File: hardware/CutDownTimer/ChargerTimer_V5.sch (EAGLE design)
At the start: 50 parts, among them Q1 2N3906, Q3 2N3906, Q4 2N3906, T1 2N3904, T2 2N3904, T4 2N3904, U1 ADCMP354OC, U2 ADCMP354OC, U3 LM60

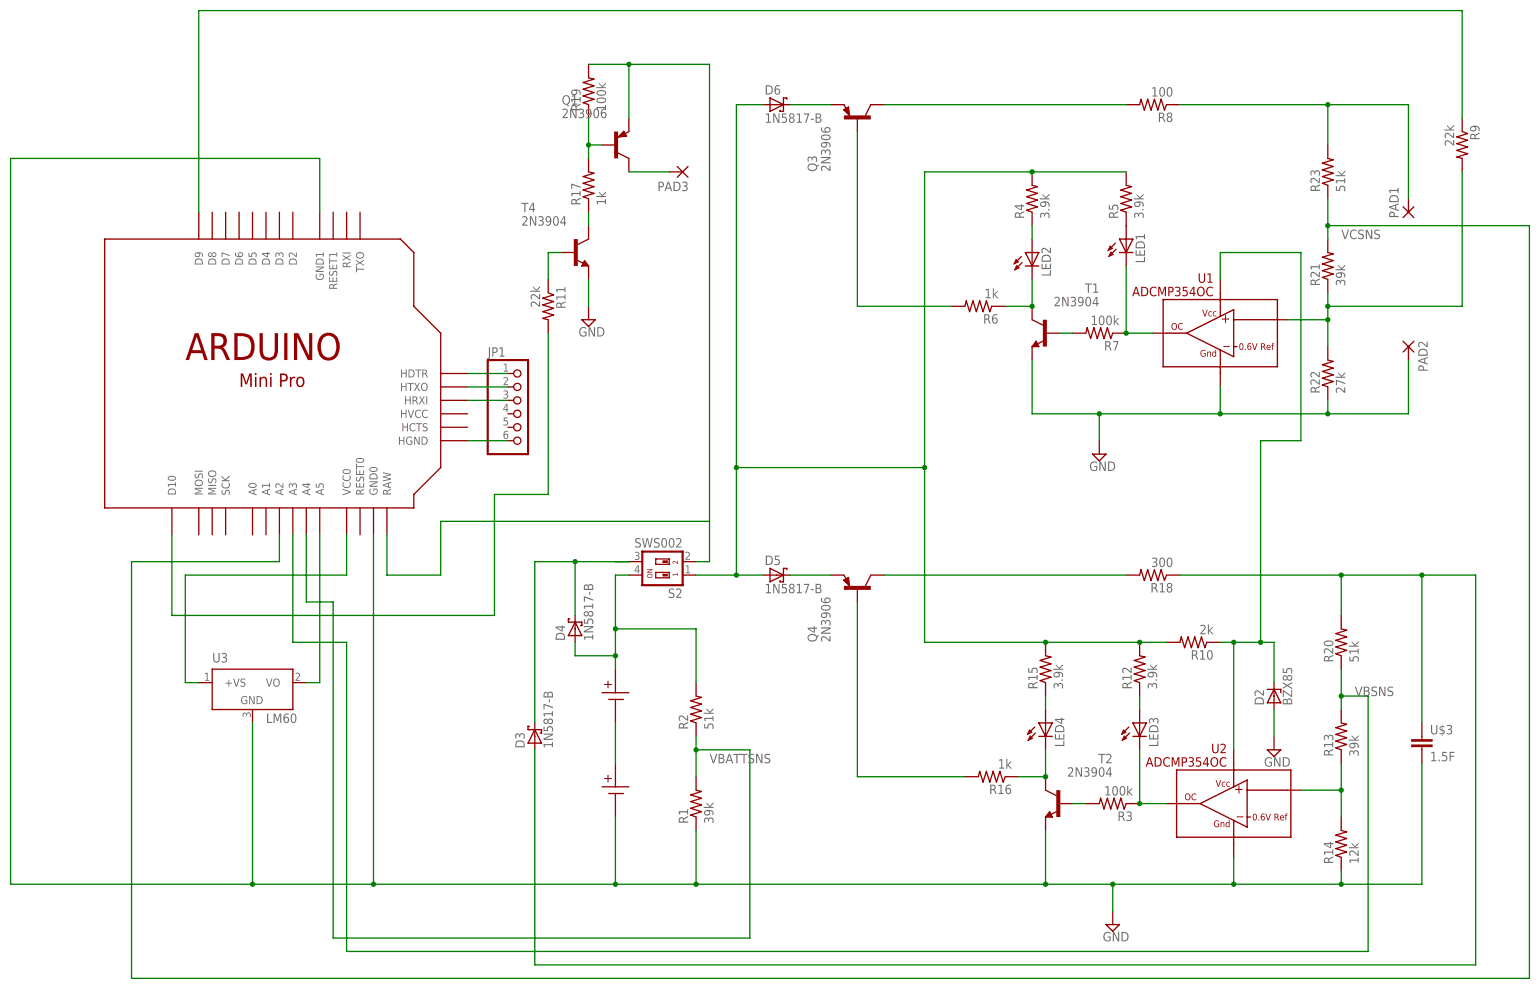
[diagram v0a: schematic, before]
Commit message: Updates
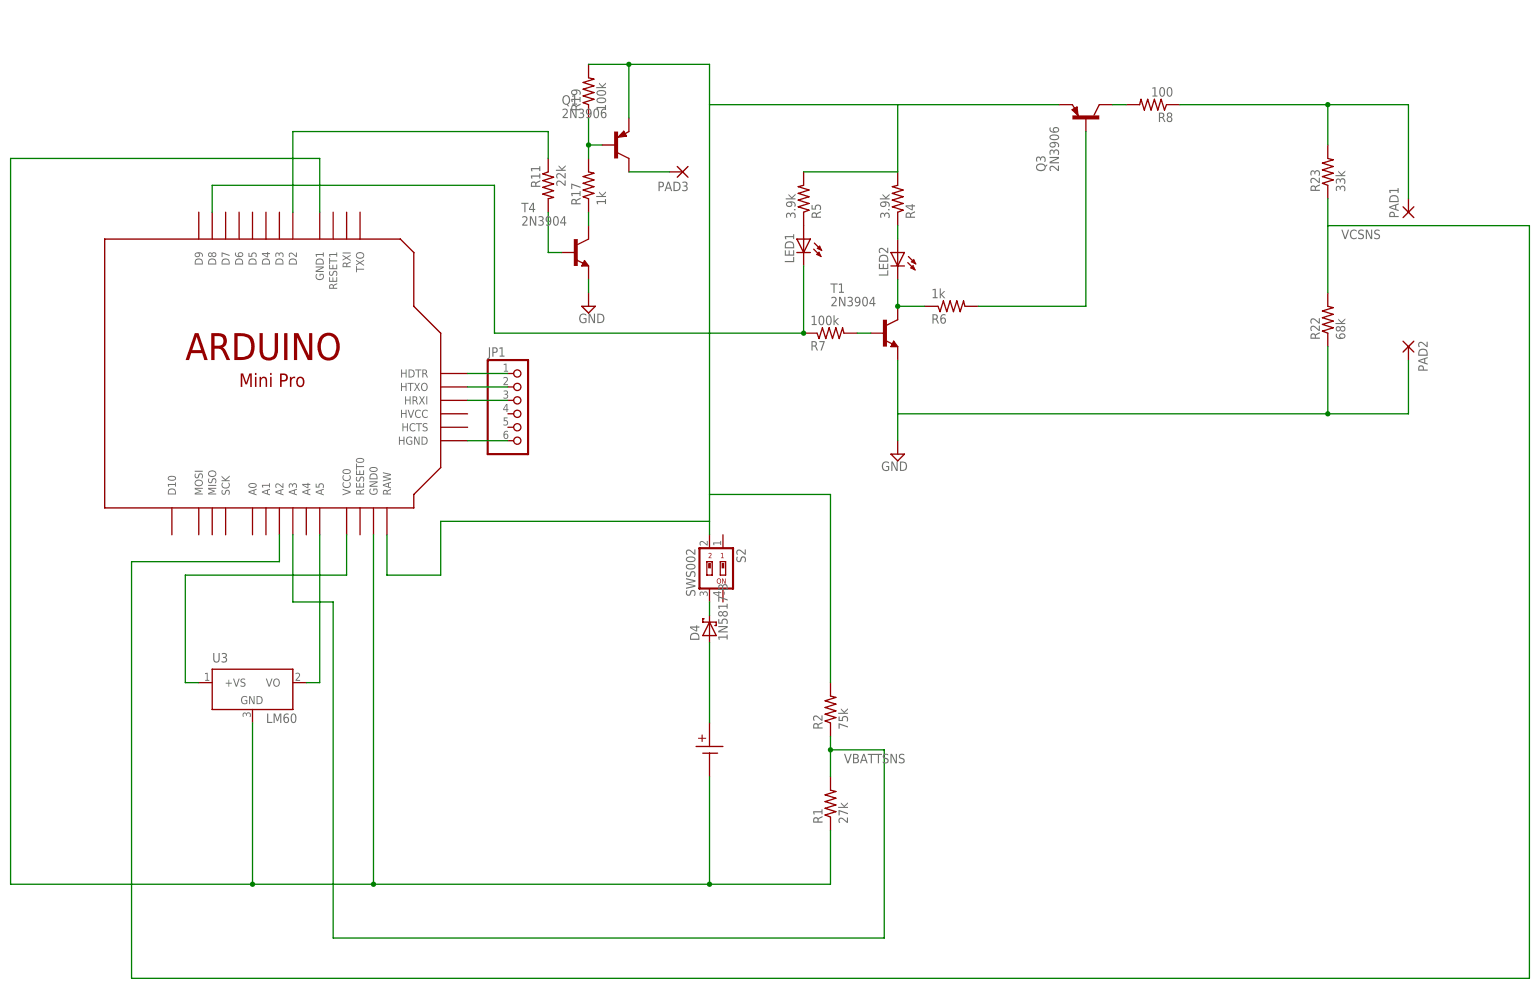
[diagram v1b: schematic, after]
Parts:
- removed D2: BZX85, diode:BZX85
- removed D3, D5, D6: 1N5817-B, diode:1N5817-B
- removed LED3, LED4: (no value), eagle-ltspice:LED_ELD260
- removed Q4: 2N3906, transistor-pnp:2N3906
- removed R10: 2k, rcl:R-US_0207/7
- removed R12, R15: 3.9k, rcl:R-US_0207/7
- removed R13, R21: 39k, rcl:R-US_0207/7
- removed R14: 12k, rcl:R-US_0207/7
- removed R16: 1k, rcl:R-US_0207/7
- removed R18: 300, rcl:R-US_0207/7
- removed R20: 51k, rcl:R-US_0207/7
- removed R3: 100k, rcl:R-US_0207/7
- removed R9: 22k, rcl:R-US_0207/7
- removed T2: 2N3904, transistor:2N3904
- removed U$2: BH1000G, mymechanical:BH1000G
- removed U$3: 1.5F, mypassives:C1000X850
- removed U1, U2: ADCMP354OC, mydevices:ADCMP354OC
- R1: value 39k -> 27k
- R2: value 51k -> 75k
- R22: value 27k -> 68k
- R23: value 51k -> 33k
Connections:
- removed net N$1: U1.IN
- removed net N$12: U$1.P2, U$2.P1
- removed net N$14: D6.C, Q3.E
- removed net N$15: D2.C, R10.1, U1.VCC, U2.VCC
- removed net N$16: R13.1, R14.2, U2.IN
- removed net N$17: LED3.C, R3.1, U2.OUT
- removed net N$18: LED3.A, R12.1
- removed net N$19: LED4.A, R15.1
- removed net N$20: LED4.C, R16.1, T2.C
- removed net N$23: Q4.B, R16.2
- removed net N$26: R11.2, U$4.D10
- removed net N$27: Q4.C, R18.2
- removed net N$28: D5.C, Q4.E
- removed net N$34: R21.1, R22.2, R9.2
- removed net N$36: D5.A, D6.A, R10.2, R12.2, R15.2, R4.2, R5.2, S2.1
- removed net N$42: Q1.E, R19.2, S2.2, U$4.RAW
- removed net VBSNS: R13.2, R20.1, U$4.A3
- new net N$37: R1.1, U$1.P2, U$4.GND0, U$4.GND1, U3.GND
- net GND: no longer D2.A, PAD2.P, R1.1, R14.1, R22.1, T2.E, U$2.P2, U$3.2, U$4.GND0, U$4.GND1, U1.GND, U2.GND, U3.GND
- net N$10: now also R11.1, U$4.D2; no longer D3.A, R18.1, R20.2, U$3.1
- net N$11: now also Q1.E, Q3.E, R19.2, R2.2, R4.2, R5.2, S2.2, U$4.RAW; no longer D3.C, D4.C, S2.3
- net N$3: now also U$4.D8; no longer U1.OUT
- net N$31: now also R11.2; no longer R11.1
- net N$38: no longer R2.2, S2.4
- net N$8: now also D4.C, S2.3; no longer R9.1, U$4.D9
- net N$9: now also PAD2.P, R22.1; no longer R3.2, T2.B
- net VBATTSNS: now also U$4.A3; no longer U$4.A4
- net VCSNS: now also R22.2; no longer R21.2
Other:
- moved on the sheet: D4, LED1, LED2, Q3, R1, R11, R2, R22, R4, R5, R6, R7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
